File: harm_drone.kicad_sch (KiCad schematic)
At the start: 1 part, among them IC2 Microcontroller

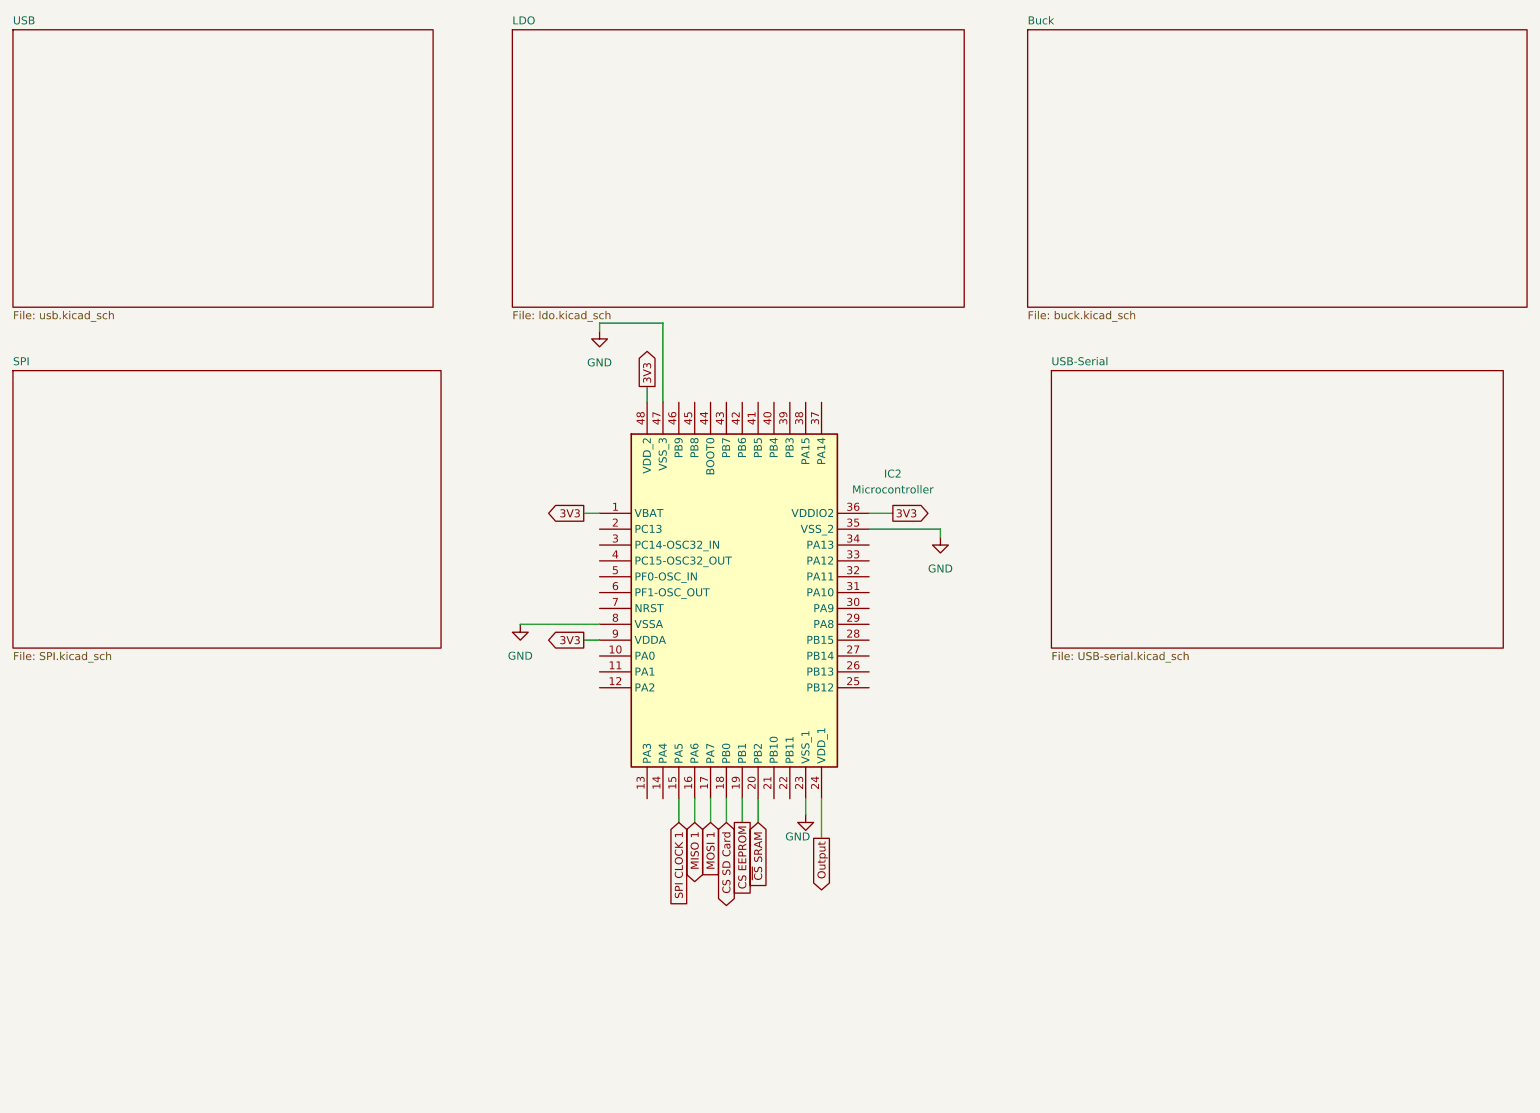
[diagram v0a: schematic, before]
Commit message: finished up schematic
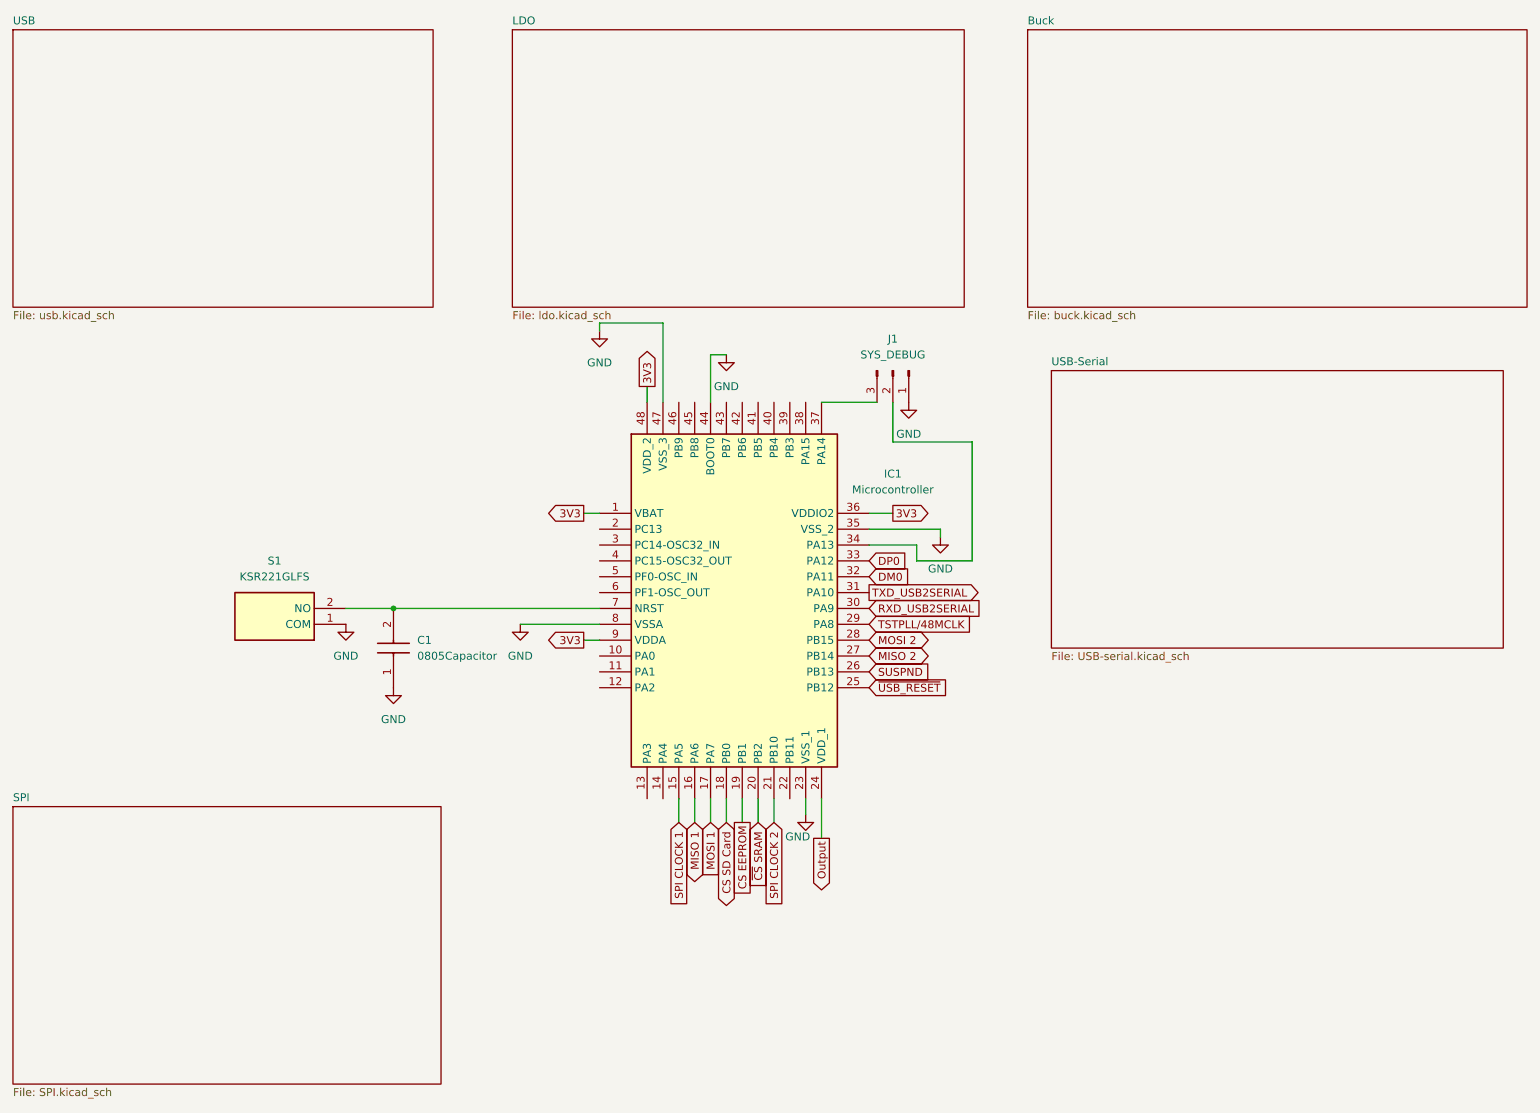
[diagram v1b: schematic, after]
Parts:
- added C1: 0805Capacitor, Capacitor_SMD:C_0805_2012Metric, symbol group127:0805Capacitor
- added J1: SYS_DEBUG, symbol Connector:Conn_01x03_Pin
- added S1: KSR221GLFS, symbol group127:KSR221GLFS
- IC1: renamed from IC2; footprint QFP50P900X900X160-48N -> (none)
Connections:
- net GND: now also IC1.44 (BOOT0), C1.1, J1.1 (Pin_1), S1.1 (COM)
- net SPI CLOCK 2: now reaches IC1.21 (PB10)
- net ~{USB_RESET}: now reaches IC1.25 (PB12)
- net SUSPND: now reaches IC1.26 (PB13)
- net MISO 2: now reaches IC1.27 (PB14)
- net MOSI 2: now reaches IC1.28 (PB15)
- net TSTPLL/48MCLK: now reaches IC1.29 (PA8)
- net RXD_USB2SERIAL: now reaches IC1.30 (PA9)
- net TXD_USB2SERIAL: now reaches IC1.31 (PA10)
- net DM0: now reaches IC1.32 (PA11)
- net DP0: now reaches IC1.33 (PA12)
- net at IC1.34 (PA13): now also J1.2 (Pin_2)
- net at IC1.37 (PA14): now also J1.3 (Pin_3)
- net at IC1.7 (NRST): now also C1.2, S1.2 (NO)
